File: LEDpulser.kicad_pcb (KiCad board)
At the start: 2 copper layers, 38.2 x 98.2 mm, 61 parts, among them J1 RJHSE5380, J2 EPS.00.250.NTN, J3 EPS.00.250.NTN, J4 Conn_01x04_Female, J5 LED, Q1 AO3401A, Q2 AO3400A, Q3 AO3400A, SW1 ATE1D-5M3-10-Z, U1 74HC123, U10 LT3082, U2 74HC123, U3 74HC123, U4 74HC10, U5 LT1121-5, U6 PM8834, U7 NE555, U8 PM8834, U9 PM8834

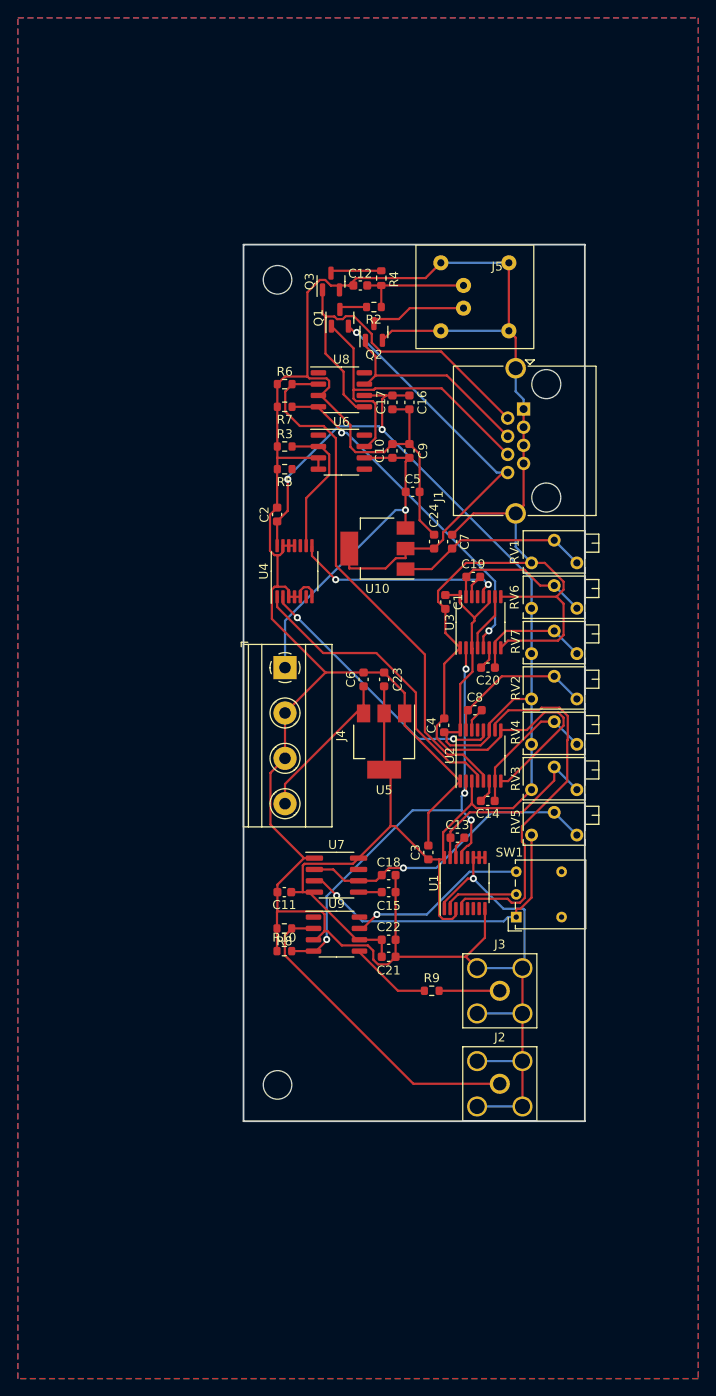
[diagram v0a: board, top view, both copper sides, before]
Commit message: reverting back to last commit
hopefuly reverting back to last commit pls
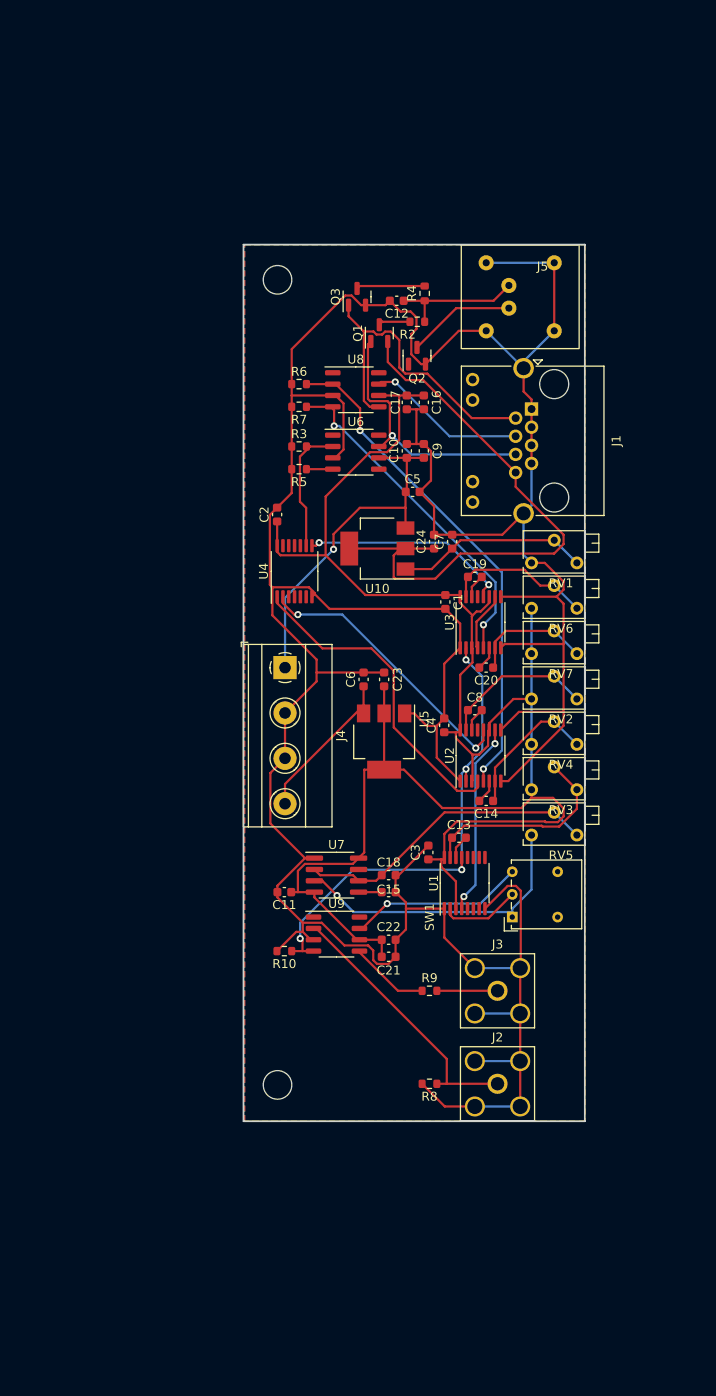
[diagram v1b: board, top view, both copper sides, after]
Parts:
- J1: value RJHSE5380 -> RJ45_Shielded; footprint Connector_RJ:RJ45_Amphenol_RJHSE5380 -> Connector_RJ:RJ45_Amphenol_RJHSE538X
- R8: value 100k -> 50
- moved R8 23.8 mm to (122.3, 119.4)
- moved Q2 5.51 mm to (120.9, 37.8)
- moved R4 5.15 mm to (121.8, 30.9)
- moved R2 5.13 mm to (120.9, 34.0)
- moved J5 5.08 mm to (132.5, 31.2)
- moved Q1 4.73 mm to (116.7, 35.3)
- moved C12 4.43 mm to (118.6, 31.7)
- moved Q3 3.39 mm to (114.2, 31.2)
- moved U6 1.61 mm to (114.0, 48.6)
- moved U8 1.61 mm to (114.0, 41.7)
- moved C10 1.61 mm to (119.8, 48.5)
- moved C16 1.61 mm to (121.7, 43.1)
- moved C17 1.61 mm to (119.8, 43.1)
- moved C9 1.61 mm to (121.7, 48.5)
- moved R3 1.61 mm to (107.7, 48.0)
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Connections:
- Q2 pad 1: /LED_ON -> unconnected-(Q2-Pad1)
- U1 pad 10: GND -> (no net)
- U1 pad 11: GND -> (no net)
- U1 pad 12: unconnected-(U1-Pad12) -> (no net)
- U1 pad 5: unconnected-(U1-Pad5) -> (no net)
- U1 pad 6: unconnected-(U1-Pad6) -> (no net)
- U1 pad 7: unconnected-(U1-Pad7) -> (no net)
- U1 pad 9: GND -> (no net)
- U4 pad 10: unconnected-(U4-Pad10) -> (no net)
- U4 pad 11: GND -> (no net)
- U4 pad 12: GND -> (no net)
- U4 pad 13: GND -> (no net)
- U4 pad 3: GND -> (no net)
- U4 pad 4: GND -> (no net)
- U4 pad 5: GND -> (no net)
- U4 pad 6: unconnected-(U4-Pad6) -> (no net)
- U6 pad 4: GND -> Net-(R5-Pad1)
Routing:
- net GND: track 438.8 -> 410.9 mm, vias 1 -> 0
- net Net-(U1-Pad4): track 41.0 -> 21.6 mm, vias 0 -> 2
- net /CAP_VOLTAGE: track 50.1 -> 65.7 mm, vias 1 -> 0
- net +5V: track 195.5 -> 207.9 mm, vias 2 -> 0
- net /CAP_CHARGE: track 37.7 -> 29.7 mm, vias 0 -> 1
- net /LED_ON: track 23.7 -> 17.9 mm, vias 0 -> 1
- net /EXT: track 35.8 -> 30.6 mm
- net /LED_SHORT: track 41.5 -> 36.5 mm
- net Net-(R6-Pad1): track 59.5 -> 56.3 mm, vias 0 -> 2
- net Net-(R5-Pad1): track 0.00 -> 2.95 mm
- net +12V: track 37.0 -> 39.5 mm
- net Net-(U2-Pad4): track 34.4 -> 36.5 mm
- net Net-(Q3-Pad3): track 5.90 -> 7.68 mm
- net Net-(C12-Pad1): track 13.2 -> 14.8 mm
- net Net-(C13-Pad1): track 22.0 -> 23.4 mm
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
